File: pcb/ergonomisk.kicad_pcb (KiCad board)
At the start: 2 copper layers, 143.5 x 119.6 mm, 22 parts

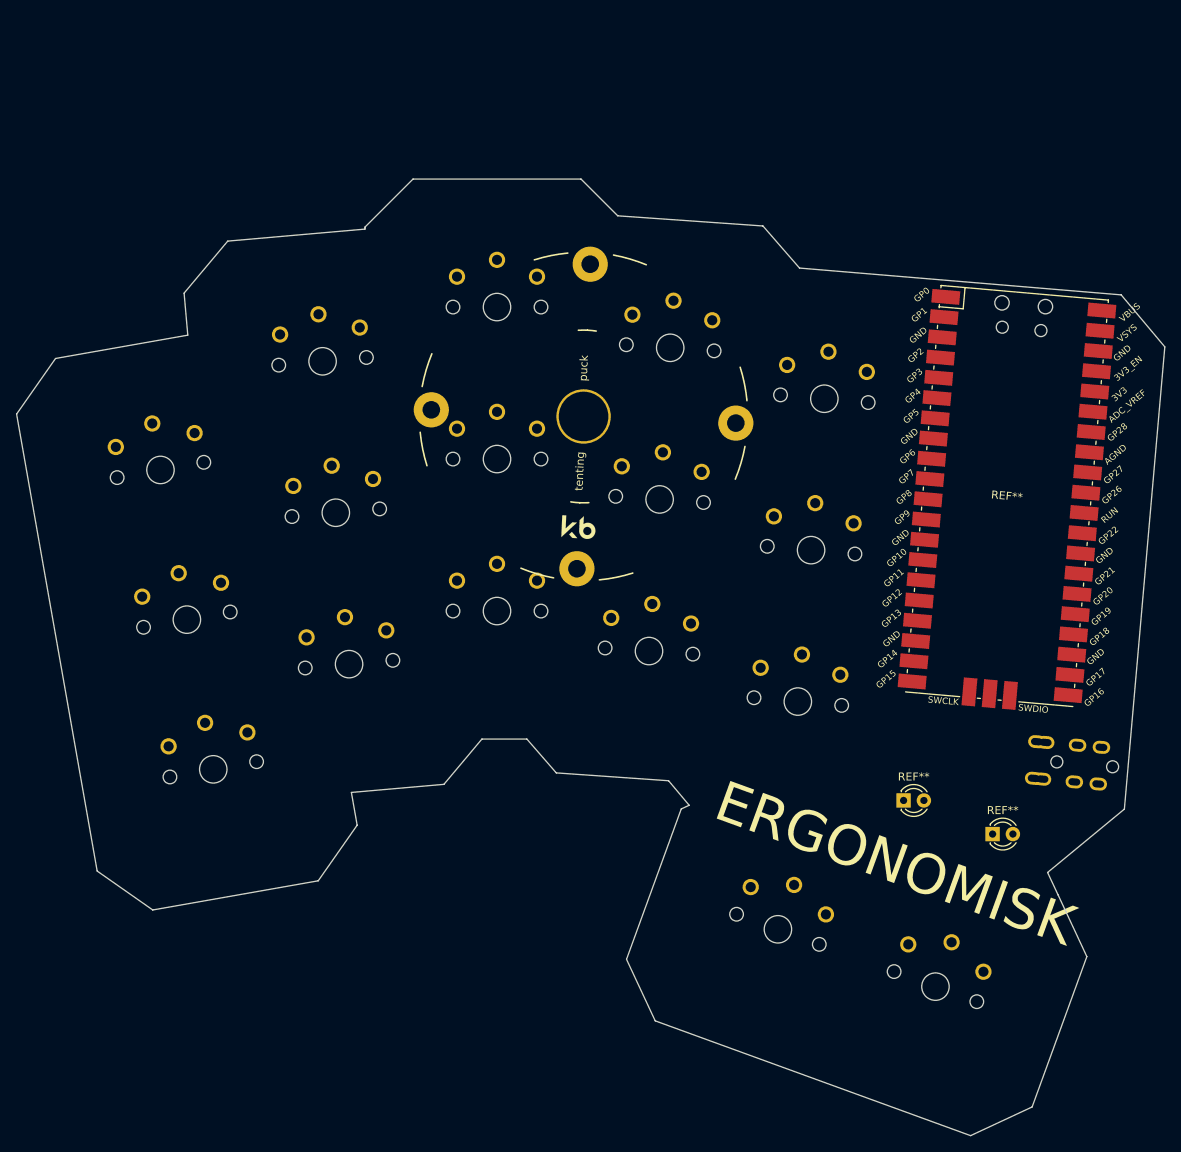
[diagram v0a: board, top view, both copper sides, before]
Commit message: feat: getting close
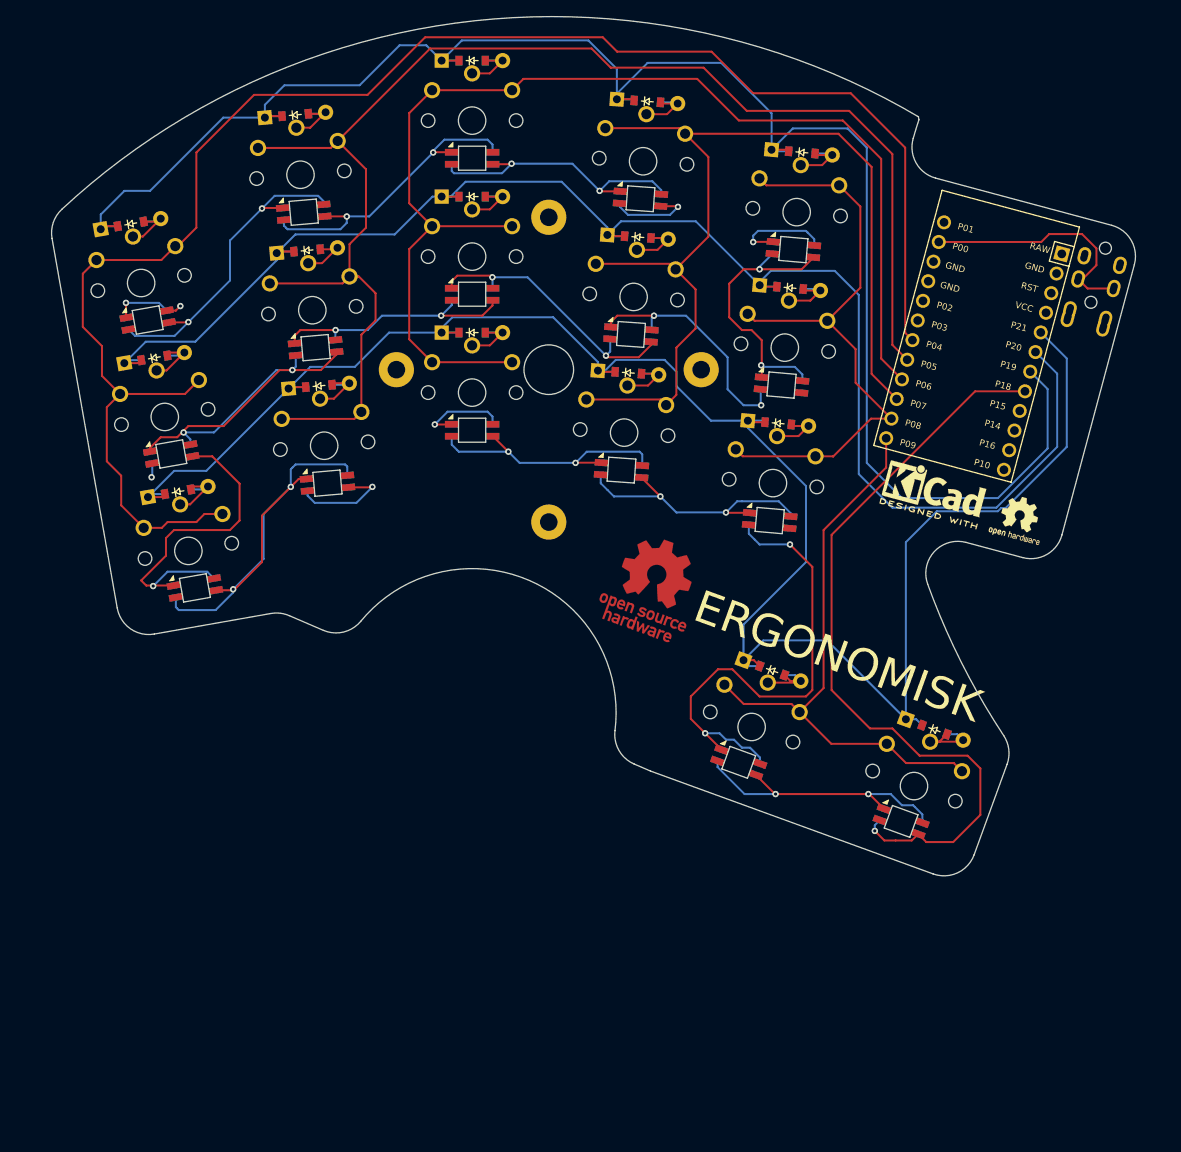
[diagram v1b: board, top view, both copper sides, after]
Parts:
- removed the REF** at (189.4, 131.2)
- removed the REF** at (200.5, 135.4)
- removed the REF** at (149.4, 83.2)
- removed the REF** at (202.3, 93.1)
- removed TRRSe: TRRS-PJ-320A-dual, TRRS-PJ-320A-dual
- added D1: , ComboDiode, F.Cu at (98.7, 92.6)
- added D10: , ComboDiode, F.Cu at (155.0, 77.7)
- added D11: , ComboDiode, F.Cu at (156.2, 60.8)
- added D12: , ComboDiode, F.Cu at (157.4, 43.8)
- added D13: , ComboDiode, F.Cu at (173.7, 84.1)
- added D14: , ComboDiode, F.Cu at (175.2, 67.1)
- added D15: , ComboDiode, F.Cu at (176.7, 50.2)
- added D16: , ComboDiode, F.Cu at (173.0, 115.0)
- added D17: , ComboDiode, F.Cu at (193.3, 122.4)
- added D2: , ComboDiode, F.Cu at (95.7, 75.9)
- added D3: , ComboDiode, F.Cu at (92.8, 59.1)
- added D4: , ComboDiode, F.Cu at (116.3, 79.4)
- added D5: , ComboDiode, F.Cu at (114.8, 62.4)
- added D6: , ComboDiode, F.Cu at (113.4, 45.5)
- added D7: , ComboDiode, F.Cu at (135.5, 72.7)
- added D8: , ComboDiode, F.Cu at (135.5, 55.7)
- added D9: , ComboDiode, F.Cu at (135.5, 38.7)
- added LED1: , SK6812MINIE, F.Cu at (100.8, 104.6)
- added LED10: , SK6812MINIE, F.Cu at (154.1, 89.9)
- added LED11: , SK6812MINIE, F.Cu at (155.3, 72.9)
- added LED12: , SK6812MINIE, F.Cu at (156.5, 56.0)
- added LED13: , SK6812MINIE, F.Cu at (172.7, 96.2)
- added LED14: , SK6812MINIE, F.Cu at (174.1, 79.3)
- added LED15: , SK6812MINIE, F.Cu at (175.6, 62.3)
- added LED16: , SK6812MINIE, F.Cu at (168.8, 126.4)
- added LED17: , SK6812MINIE, F.Cu at (189.1, 133.8)
- added LED2: , SK6812MINIE, F.Cu at (97.9, 87.9)
- added LED3: , SK6812MINIE, F.Cu at (94.9, 71.1)
- added LED4: , SK6812MINIE, F.Cu at (117.4, 91.5)
- added LED5: , SK6812MINIE, F.Cu at (115.9, 74.6)
- added LED6: , SK6812MINIE, F.Cu at (114.4, 57.7)
- added LED7: , SK6812MINIE, F.Cu at (135.5, 84.9)
- added LED8: , SK6812MINIE, F.Cu at (135.5, 67.9)
- added LED9: , SK6812MINIE, F.Cu at (135.5, 50.9)
- added MCU1: , ProMicro, F.Cu at (198.2, 74.4)
- added REF**: OSHW-Logo2_7.3x6mm_SilkScreen, Symbol:OSHW-Logo2_7.3x6mm_SilkScreen, F.Cu at (203.8, 96.0)
- added REF**: KiCad-Logo2_5mm_SilkScreen, Symbol:KiCad-Logo2_5mm_SilkScreen, F.Cu at (193.2, 92.8)
- added REF**: OSHW-Logo_11.4x12mm_Copper, Symbol:OSHW-Logo_11.4x12mm_Copper, F.Cu at (158.0, 104.4)
- added REF**: Tenting Puck, TENTINGPUCK, F.Cu at (145.1, 77.3)
- added TRRS1: TRRS-PJ-320A-dual, TRRS-PJ-320A-dual, F.Cu at (217.3, 61.2)
- S1, S10, S11, S12, S13, S14, S15, S16, S17, S2, S3, S4, S5, S6, S7, S8, S9: footprint ergonomisk:PG1350 -> PG1350
- moved S1 27.5 mm to (100.0, 100.0)
- moved S10 27.5 mm to (154.5, 85.2)
- moved S13 27.5 mm to (173.1, 91.5)
- moved S4 27.5 mm to (117.0, 86.9)
- moved S7 27.5 mm to (135.5, 80.2)
- moved S14 25.5 mm to (174.6, 74.6)
- moved S11 25.5 mm to (155.7, 68.3)
- moved S16 25.5 mm to (170.4, 122.0)
- moved S8 25.5 mm to (135.5, 63.2)
- moved S2 25.5 mm to (97.0, 83.3)
- moved S5 25.5 mm to (115.5, 69.9)
- moved S17 25.2 mm to (190.7, 129.4)
- moved S15 23.6 mm to (176.0, 57.7)
- moved S12 23.6 mm to (156.8, 51.3)
- moved S9 23.5 mm to (135.5, 46.2)
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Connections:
- S1 pad 1: GND -> P4
- S1 pad 2: (no net) -> pinky_bottom
- S10 pad 1: GND -> P7
- S10 pad 2: (no net) -> index_bottom
- S11 pad 1: GND -> P7
- S11 pad 2: (no net) -> index_home
- S12 pad 1: GND -> P7
- S12 pad 2: (no net) -> index_top
- S13 pad 1: GND -> P8
- S13 pad 2: (no net) -> far_bottom
- S14 pad 1: GND -> P8
- S14 pad 2: (no net) -> far_home
- S15 pad 1: GND -> P8
- S15 pad 2: (no net) -> far_top
- S16 pad 1: GND -> P9
- S16 pad 2: (no net) -> inner_keys
- S17 pad 1: GND -> P9
- S17 pad 2: (no net) -> outer_keys
- S2 pad 1: GND -> P4
- S2 pad 2: (no net) -> pinky_home
- S3 pad 1: GND -> P4
- S3 pad 2: (no net) -> pinky_top
- S4 pad 1: GND -> P5
- S4 pad 2: (no net) -> ring_bottom
- S5 pad 1: GND -> P5
- S5 pad 2: (no net) -> ring_home
- S6 pad 1: GND -> P5
- S6 pad 2: (no net) -> ring_top
- S7 pad 1: GND -> P6
- S7 pad 2: (no net) -> middle_bottom
- S8 pad 1: GND -> P6
- S8 pad 2: (no net) -> middle_home
- S9 pad 1: GND -> P6
- S9 pad 2: (no net) -> middle_top
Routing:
- net P21: track 0.00 -> 246.4 mm
- net P19: track 0.00 -> 225.1 mm
- net P4: track 0.00 -> 208.1 mm
- net P20: track 0.00 -> 198.6 mm
- net P5: track 0.00 -> 176.0 mm
- net P6: track 0.00 -> 148.2 mm
- net P7: track 0.00 -> 125.5 mm
- net P18: track 0.00 -> 96.9 mm, vias 0 -> 1
- net P8: track 0.00 -> 77.7 mm
- net P9: track 0.00 -> 72.9 mm
- net thumb_near_dout: track 0.00 -> 61.6 mm, vias 0 -> 2
- net bot_ring_dout: track 0.00 -> 56.8 mm, vias 0 -> 2
- net home_pinky_dout: track 0.00 -> 49.6 mm, vias 0 -> 2
- net bot_pinky_dout: track 0.00 -> 43.4 mm, vias 0 -> 2
- net top_ring_dout: track 0.00 -> 40.7 mm, vias 0 -> 2
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- added copper zone on In1.Cu, net GND
- added copper zone on In2.Cu, net RAW
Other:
- board size 143.5 x 119.6 mm -> 135.5 x 107.4 mm
- copper layers 2 -> 4
